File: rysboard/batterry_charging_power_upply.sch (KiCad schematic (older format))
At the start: 27 parts, among them J20 Conn_01x02, Q16 NST847BDP6T5G, Q5 DMP3036SSD-13, Q6 DMP3036SSD-13, Q9 Si7938DP-T1-GE3, U12 LTC4007

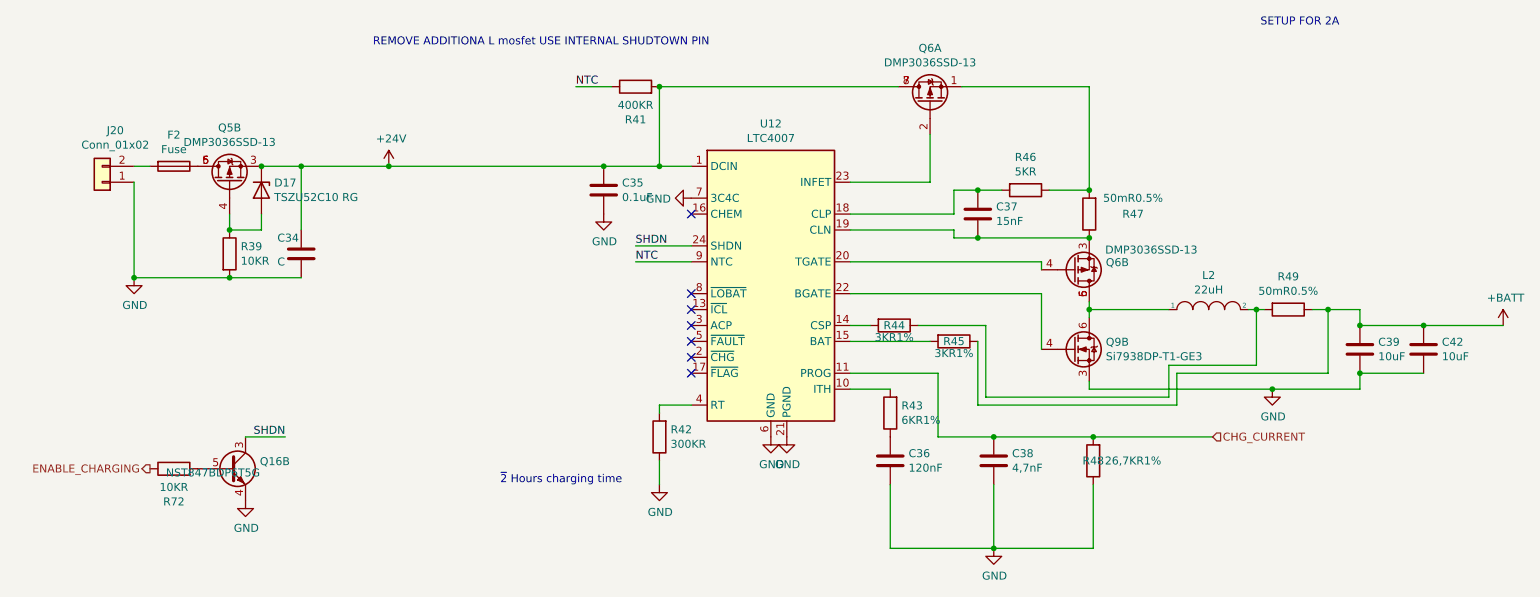
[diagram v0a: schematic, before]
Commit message: cleanup and energy managment scheeme started
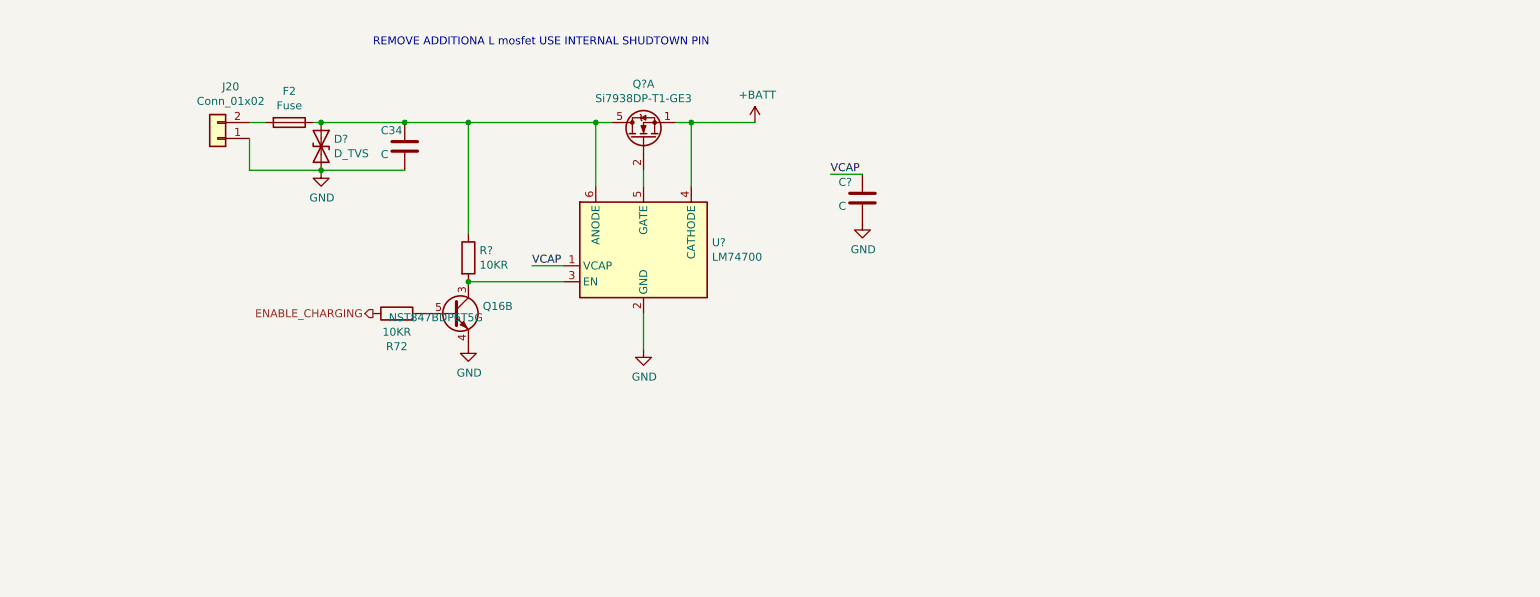
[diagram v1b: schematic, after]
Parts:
- removed C35: 0.1uF, Capacitor_SMD:C_0603_1608Metric, symbol Device:C
- removed C36: 120nF, Capacitor_SMD:C_0603_1608Metric, symbol Device:C
- removed C37: 15nF, Capacitor_SMD:C_0603_1608Metric, symbol Device:C
- removed C38: 4,7nF, Capacitor_SMD:C_0603_1608Metric_Pad1.05x0.95mm_HandSolder, symbol Device:C
- removed C39, C42: 10uF, Capacitor_SMD:C_1206_3216Metric, symbol Device:C
- removed D17: TSZU52C10 RG, Diode_SMD:D_0603_1608Metric, symbol Device:D_Zener
- removed L2: 22uH, Inductor_SMD:L_10.4x10.4_H4.8, symbol pspice:INDUCTOR
- removed Q5, Q6: DMP3036SSD-13, Package_SO:SO-8_3.9x4.9mm_P1.27mm, symbol rysboard:DMP3036SSD-13
- removed Q9: Si7938DP-T1-GE3, Package_SO:PowerPAK_SO-8_Dual, symbol rysboard:Si7938DP-T1-GE3
- removed R39: 10KR, Resistor_SMD:R_0603_1608Metric_Pad1.05x0.95mm_HandSolder, symbol Device:R
- removed R41: 400KR, Resistor_SMD:R_0603_1608Metric, symbol Device:R
- removed R42: 300KR, Resistor_SMD:R_0603_1608Metric_Pad1.05x0.95mm_HandSolder, symbol Device:R
- removed R43: 6KR1%, Resistor_SMD:R_0603_1608Metric, symbol Device:R
- removed R44, R45: 3KR1%, Resistor_SMD:R_0603_1608Metric, symbol Device:R
- removed R46: 5KR, Resistor_SMD:R_0603_1608Metric_Pad1.05x0.95mm_HandSolder, symbol Device:R
- removed R47, R49: 50mR0.5%, Resistor_SMD:R_1206_3216Metric, symbol Device:R
- removed R48: 26,7KR1%, Resistor_SMD:R_0603_1608Metric, symbol Device:R
- removed U12: LTC4007, Package_SO:SSOP-24_3.9x8.7mm_P0.635mm, symbol Battery_Management:LTC4007
- added C?: C, Capacitor_SMD:C_0603_1608Metric, symbol Device:C
- added D?: D_TVS, symbol Device:D_TVS
- added Q?: Si7938DP-T1-GE3, Package_SO:PowerPAK_SO-8_Dual, symbol rysboard:Si7938DP-T1-GE3
- added R?: 10KR, Resistor_SMD:R_0603_1608Metric_Pad1.05x0.95mm_HandSolder, symbol Device:R
- added U?: LM74700, Package_TO_SOT_SMD:SOT-23-6, symbol Power_Management:LM74700
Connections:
- net +24V is gone; now on an unnamed net: C34.1
- net +BATT: now also Q?.1 (S1), U?.4 (CATHODE)
- net GND: now also C?.2, D?.2 (A2), U?.2 (GND)
- net at F2.1: now also D?.1 (A1), Q?.5 (D1), R?.1, U?.6 (ANODE)
- net SHDN: no longer names the net of Q16.3 (C2)
- net SHDN: now also R?.2, U?.3 (EN)
- new net: Q?.2 (G1), U?.5 (GATE)
- new net VCAP: C?.1, U?.1 (VCAP)
- no-connect marks 7 -> 0
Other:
- note removed: "SETUP FOR 2A"
- note removed: "~2 Hours charging time"
- moved on the sheet: C34, F2, J20, Q16B, R72

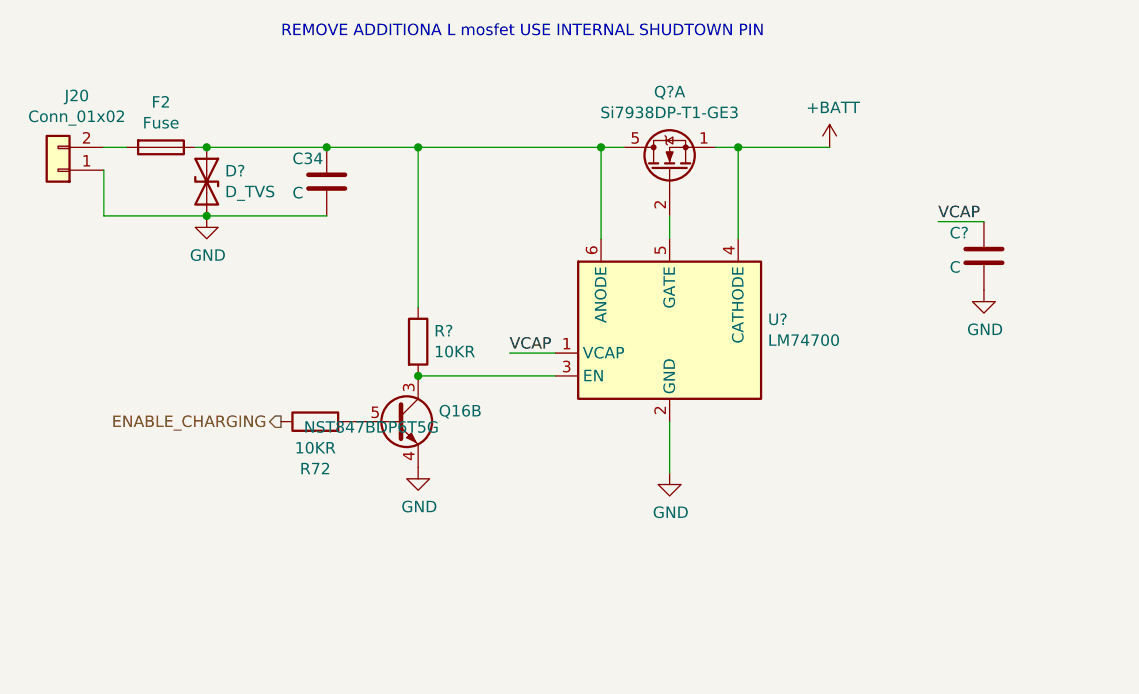
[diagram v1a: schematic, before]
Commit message: started board project
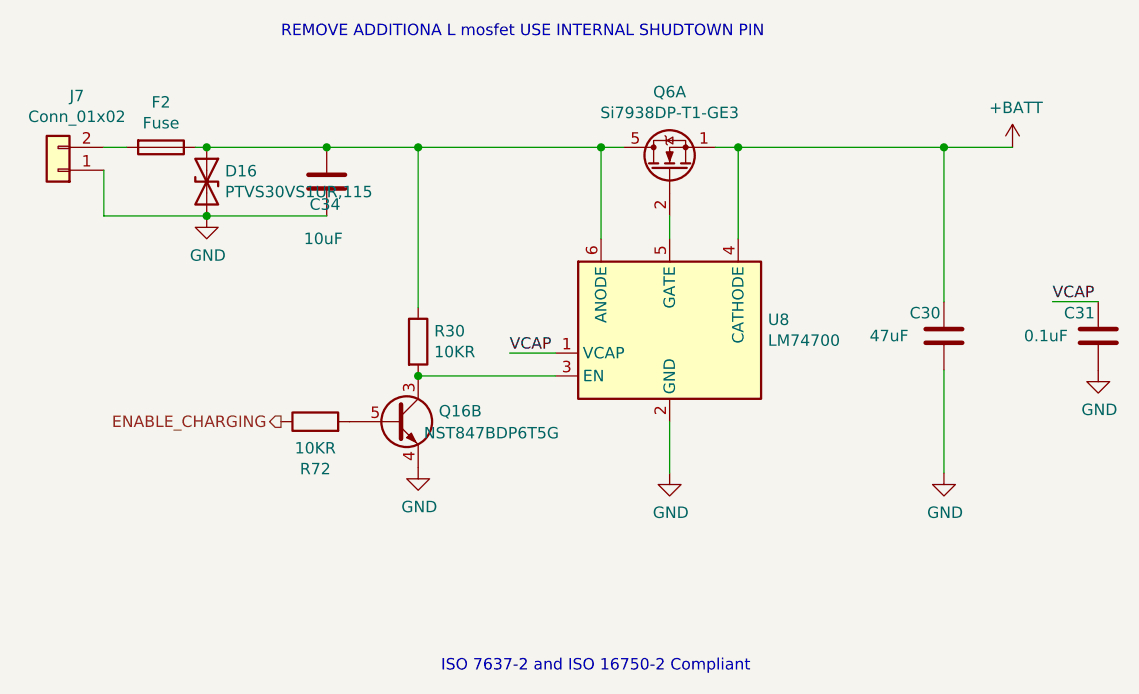
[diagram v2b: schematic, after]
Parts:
- added C30: 47uF, Capacitor_Tantalum_SMD:CP_EIA-7343-31_Kemet-D, symbol Device:C
- C31: renamed from C?; value C -> 0.1uF
- C34: value C -> 10uF; footprint Capacitor_SMD:C_0603_1608Metric -> Capacitor_SMD:C_1206_3216Metric
- D16: renamed from D?; value D_TVS -> PTVS30VS1UR,115; footprint (none) -> Diode_SMD:D_SOD-123
- F2: footprint Fuse:Fuse_1206_3216Metric -> Fuse:Fuse_2512_6332Metric
- J7: renamed from J20; footprint (none) -> Connector_Molex:Molex_Micro-Fit_3.0_43045-0212_2x01_P3.00mm_Vertical
- gave numbers to parts that had none: 3
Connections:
- net +BATT: now also C30.1
- net GND: now also C30.2
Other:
- note added: "ISO 7637-2 and ISO 16750-2 Compliant\n"
- moved on the sheet: C31
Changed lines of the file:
@@
 $EndDescr
 $Comp
-L Connector_Generic:Conn_01x02 J20
+L Connector_Generic:Conn_01x02 J7
 U 1 1 5FEFA283
 P 2075 1575
-F 0 "J20" H 1993 1250 50  0000 C CNN
+F 0 "J7" H 1993 1250 50  0000 C CNN
 F 1 "Conn_01x02" H 1993 1341 50  0000 C CNN
-F 2 "" H 2075 1575 50  0001 C CNN
+F 2 "Connector_Molex:Molex_Micro-Fit_3.0_43045-0212_2x01_P3.00mm_Vertical" H 2075 1575 50  0001 C CNN
 F 3 "~" H 2075 1575 50  0001 C CNN
 	1    2075 1575
@@
 F 0 "F2" V 2328 1475 50  0000 C CNN
 F 1 "Fuse" V 2419 1475 50  0000 C CNN
-F 2 "Fuse:Fuse_1206_3216Metric" V 2455 1475 50  0001 C CNN
+F 2 "Fuse:Fuse_2512_6332Metric" V 2455 1475 50  0001 C CNN
 F 3 "~" H 2525 1475 50  0001 C CNN
 	1    2525 1475
@@
 L power:+BATT #PWR048
 U 1 1 605BB790
-P 5450 1475
-F 0 "#PWR048" H 5450 1325 50  0001 C CNN
-F 1 "+BATT" H 5465 1648 50  0000 C CNN
-F 2 "" H 5450 1475 50  0001 C CNN
-F 3 "" H 5450 1475 50  0001 C CNN
-	1    5450 1475
+P 6250 1475
+F 0 "#PWR048" H 6250 1325 50  0001 C CNN
+F 1 "+BATT" H 6265 1648 50  0000 C CNN
+F 2 "" H 6250 1475 50  0001 C CNN
+F 3 "" H 6250 1475 50  0001 C CNN
+	1    6250 1475
 	1    0    0    -1
 $EndComp
@@
 U 1 1 6069566D
 P 3250 1625
-F 0 "C34" H 3100 1725 50  0000 L CNN
-F 1 "C" H 3100 1575 50  0000 L CNN
-F 2 "Capacitor_SMD:C_0603_1608Metric" H 3288 1475 50  0001 C CNN
+F 0 "C34" H 3175 1525 50  0000 L CNN
+F 1 "10uF" H 3150 1375 50  0000 L CNN
+F 2 "Capacitor_SMD:C_1206_3216Metric" H 3288 1475 50  0001 C CNN
 F 3 "~" H 3250 1625 50  0001 C CNN
 	1    3250 1625
@@
 P 3550 2675
 F 0 "Q16" H 3740 2721 50  0000 L CNN
-F 1 "NST847BDP6T5G" H 3150 2650 50  0000 L CNN
+F 1 "NST847BDP6T5G" H 3675 2625 50  0000 L CNN
 F 2 "Package_TO_SOT_SMD:SOT-963" H 3750 2775 50  0001 C CNN
 F 3 "~" H 3550 2675 50  0001 C CNN
@@
 $EndComp
 $Comp
-L Device:R R?
+L Device:R R30
 U 1 1 6057BE19
 P 3650 2325
-F 0 "R?" H 3720 2371 50  0000 L CNN
+F 0 "R30" H 3720 2371 50  0000 L CNN
 F 1 "10KR" H 3720 2280 50  0000 L CNN
 F 2 "Resistor_SMD:R_0603_1608Metric_Pad1.05x0.95mm_HandSolder" V 3580 2325 50  0001 C CNN
@@
 $EndComp
 $Comp
-L Power_Management:LM74700 U?
+L Power_Management:LM74700 U8
 U 1 1 6056EF72
 P 4750 2275
-F 0 "U?" H 5180 2321 50  0000 L CNN
+F 0 "U8" H 5180 2321 50  0000 L CNN
 F 1 "LM74700" H 5180 2230 50  0000 L CNN
 F 2 "Package_TO_SOT_SMD:SOT-23-6" H 4375 1925 50  0001 C CNN
@@
 	1    0    0    -1
 $EndComp
-$Comp
-L rysboard:Si7938DP-T1-GE3 Q?
+Wire Wire Line
+	4750 1775 4750 1875
+Wire Wire Line
+	4550 1475 4450 1475
+Wire Wire Line
+	4450 1475 4450 1875
+Wire Wire Line
+	4950 1475 5050 1475
+Wire Wire Line
+	5050 1475 5050 1875
+Connection ~ 5050 1475
+Connection ~ 3650 2475
+Connection ~ 4450 1475
+$Comp
+L power:GND #PWR040
+U 1 1 60572C01
+P 4750 2900
+F 0 "#PWR040" H 4750 2650 50  0001 C CNN
+F 1 "GND" H 4755 2727 50  0000 C CNN
+F 2 "" H 4750 2900 50  0001 C CNN
+F 3 "" H 4750 2900 50  0001 C CNN
+	1    4750 2900
+	1    0    0    -1
+$EndComp
+Wire Wire Line
+	4750 2900 4750 2675
+$Comp
+L Device:C C31
+U 1 1 60573158
+P 6625 2300
+F 0 "C31" H 6475 2400 50  0000 L CNN
+F 1 "0.1uF" H 6300 2300 50  0000 L CNN
+F 2 "Capacitor_SMD:C_0603_1608Metric" H 6663 2150 50  0001 C CNN
+F 3 "~" H 6625 2300 50  0001 C CNN
+	1    6625 2300
+	1    0    0    -1
+$EndComp
+Wire Wire Line
+	3650 2175 3650 1475
+Wire Wire Line
+	3650 1475 4450 1475
+Wire Wire Line
+	3650 2475 4250 2475
+$Comp
+L power:GND #PWR042
+U 1 1 60574E8B
+P 6625 2450
+F 0 "#PWR042" H 6625 2200 50  0001 C CNN
+F 1 "GND" H 6630 2277 50  0000 C CNN
+F 2 "" H 6625 2450 50  0001 C CNN
+F 3 "" H 6625 2450 50  0001 C CNN
+	1    6625 2450
+	1    0    0    -1
+$EndComp
+Text Label 4050 2375 0    50   ~ 0
+VCAP
+Wire Wire Line
+	4050 2375 4250 2375
+Text Label 6425 2150 0    50   ~ 0
+VCAP
+Wire Wire Line
+	6425 2150 6625 2150
+Wire Wire Line
+	2675 1475 2725 1475
+Wire Wire Line
+	3250 1475 3650 1475
+Connection ~ 3250 1475
+Connection ~ 3650 1475
+$Comp
+L Device:D_TVS D16
+U 1 1 6057AB93
+P 2725 1625
+F 0 "D16" V 2679 1705 50  0000 L CNN
+F 1 "PTVS30VS1UR,115 " V 2770 1705 50  0000 L CNN
+F 2 "Diode_SMD:D_SOD-123" H 2725 1625 50  0001 C CNN
+F 3 "~" H 2725 1625 50  0001 C CNN
+	1    2725 1625
+	0    1    1    0
+$EndComp
+Connection ~ 2725 1475
+Wire Wire Line
+	2725 1475 3250 1475
+Wire Wire Line
+	3250 1775 2725 1775
+Wire Wire Line
+	2275 1775 2275 1575
+Connection ~ 2725 1775
+Wire Wire Line
+	2725 1775 2275 1775
+Text Notes 3750 3775 0    50   ~ 0
+ISO 7637-2 and ISO 16750-2 Compliant\n
+$Comp
+L Device:C C30
+U 1 1 605A31DC
+P 5950 2300
+F 0 "C30" H 5800 2400 50  0000 L CNN
+F 1 "47uF" H 5625 2300 50  0000 L CNN
+F 2 "Capacitor_Tantalum_SMD:CP_EIA-7343-31_Kemet-D" H 5988 2150 50  0001 C CNN
+F 3 "~" H 5950 2300 50  0001 C CNN
+	1    5950 2300
+	1    0    0    -1
+$EndComp
+Wire Wire Line
+	6250 1475 5950 1475
+Wire Wire Line
+	5950 1475 5950 2150
+Wire Wire Line
+	5050 1475 5950 1475
+Connection ~ 5950 1475
+$Comp
+L power:GND #PWR041
+U 1 1 605ADEA3
+P 5950 2900
+F 0 "#PWR041" H 5950 2650 50  0001 C CNN
+F 1 "GND" H 5955 2727 50  0000 C CNN
+F 2 "" H 5950 2900 50  0001 C CNN
+F 3 "" H 5950 2900 50  0001 C CNN
+	1    5950 2900
+	1    0    0    -1
+$EndComp
+Wire Wire Line
+	5950 2900 5950 2450
+$Comp
+L rysboard:Si7938DP-T1-GE3 Q6
 U 1 1 6056F7A8
 P 4750 1575
-F 0 "Q?" V 5092 1575 50  0000 C CNN
+F 0 "Q6" V 5092 1575 50  0000 C CNN
 F 1 "Si7938DP-T1-GE3" V 5001 1575 50  0000 C CNN
 F 2 "Package_SO:PowerPAK_SO-8_Dual" H 4950 1500 50  0001 L CIN
@@
 	0    -1   -1   0
 $EndComp
-Wire Wire Line
-	4750 1775 4750 1875
-Wire Wire Line
-	4550 1475 4450 1475
-Wire Wire Line
-	4450 1475 4450 1875
-Wire Wire Line
-	4950 1475 5050 1475
-Wire Wire Line
-	5050 1475 5050 1875
-Wire Wire Line
-	5450 1475 5050 1475
-Connection ~ 5050 1475
-Connection ~ 3650 2475
-Connection ~ 4450 1475
-$Comp
-L power:GND #PWR?
-U 1 1 60572C01
-P 4750 2900
-F 0 "#PWR?" H 4750 2650 50  0001 C CNN
-F 1 "GND" H 4755 2727 50  0000 C CNN
-F 2 "" H 4750 2900 50  0001 C CNN
-F 3 "" H 4750 2900 50  0001 C CNN
-	1    4750 2900
-	1    0    0    -1
-$EndComp
-Wire Wire Line
-	4750 2900 4750 2675
-$Comp
-L Device:C C?
-U 1 1 60573158
-P 6125 1950
-F 0 "C?" H 5975 2050 50  0000 L CNN
-F 1 "C" H 5975 1900 50  0000 L CNN
-F 2 "Capacitor_SMD:C_0603_1608Metric" H 6163 1800 50  0001 C CNN
-F 3 "~" H 6125 1950 50  0001 C CNN
-	1    6125 1950
-	1    0    0    -1
-$EndComp
-Wire Wire Line
-	3650 2175 3650 1475
-Wire Wire Line
-	3650 1475 4450 1475
-Wire Wire Line
-	3650 2475 4250 2475
-$Comp
-L power:GND #PWR?
-U 1 1 60574E8B
-P 6125 2100
-F 0 "#PWR?" H 6125 1850 50  0001 C CNN
-F 1 "GND" H 6130 1927 50  0000 C CNN
-F 2 "" H 6125 2100 50  0001 C CNN
-F 3 "" H 6125 2100 50  0001 C CNN
-	1    6125 2100
-	1    0    0    -1
-$EndComp
-Text Label 4050 2375 0    50   ~ 0
-VCAP
-Wire Wire Line
-	4050 2375 4250 2375
-Text Label 5925 1800 0    50   ~ 0
-VCAP
-Wire Wire Line
-	5925 1800 6125 1800
-Wire Wire Line
-	2675 1475 2725 1475
-Wire Wire Line
-	3250 1475 3650 1475
-Connection ~ 3250 1475
-Connection ~ 3650 1475
-$Comp
-L Device:D_TVS D?
-U 1 1 6057AB93
-P 2725 1625
-F 0 "D?" V 2679 1705 50  0000 L CNN
-F 1 "D_TVS" V 2770 1705 50  0000 L CNN
-F 2 "" H 2725 1625 50  0001 C CNN
-F 3 "~" H 2725 1625 50  0001 C CNN
-	1    2725 1625
-	0    1    1    0
-$EndComp
-Connection ~ 2725 1475
-Wire Wire Line
-	2725 1475 3250 1475
-Wire Wire Line
-	3250 1775 2725 1775
-Wire Wire Line
-	2275 1775 2275 1575
-Connection ~ 2725 1775
-Wire Wire Line
-	2725 1775 2275 1775
 $EndSCHEMATC
